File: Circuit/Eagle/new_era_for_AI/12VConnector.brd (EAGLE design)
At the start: 55.7 x 27.8 mm, 12 parts

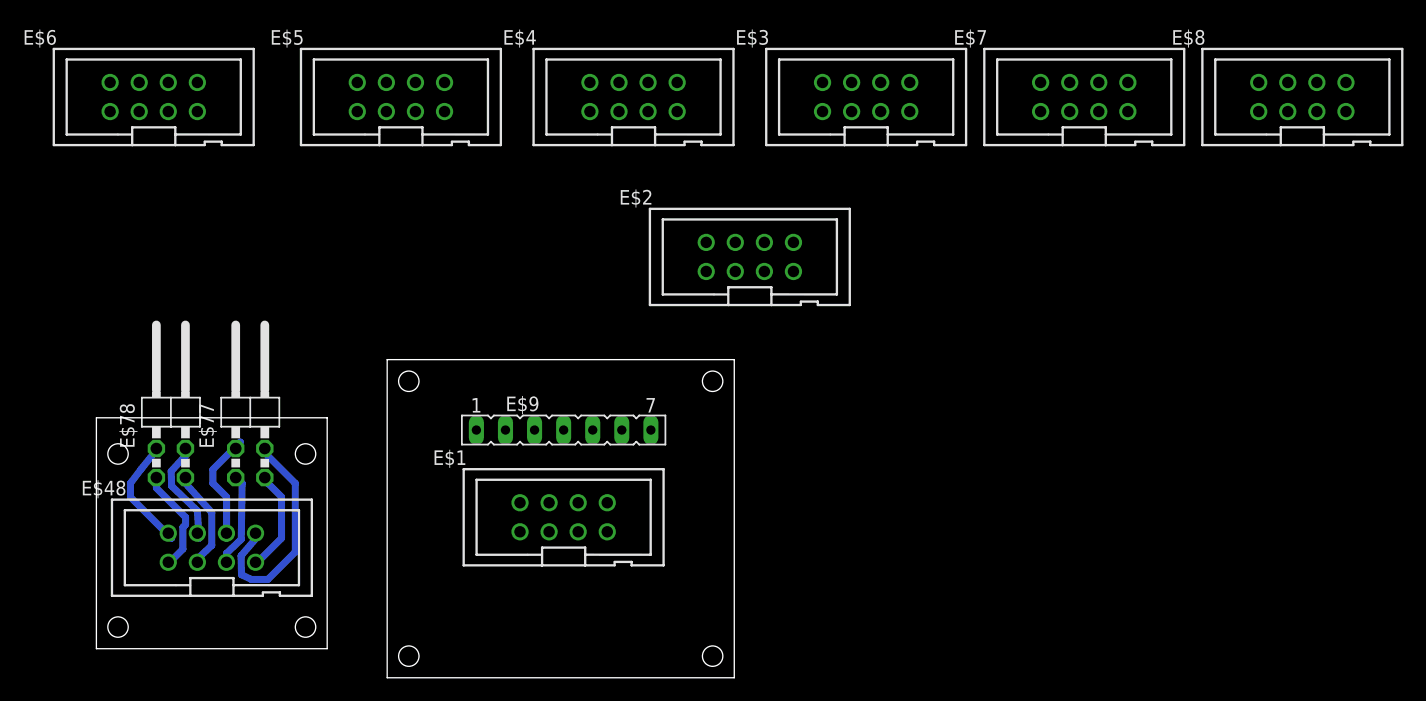
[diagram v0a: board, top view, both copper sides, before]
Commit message: .
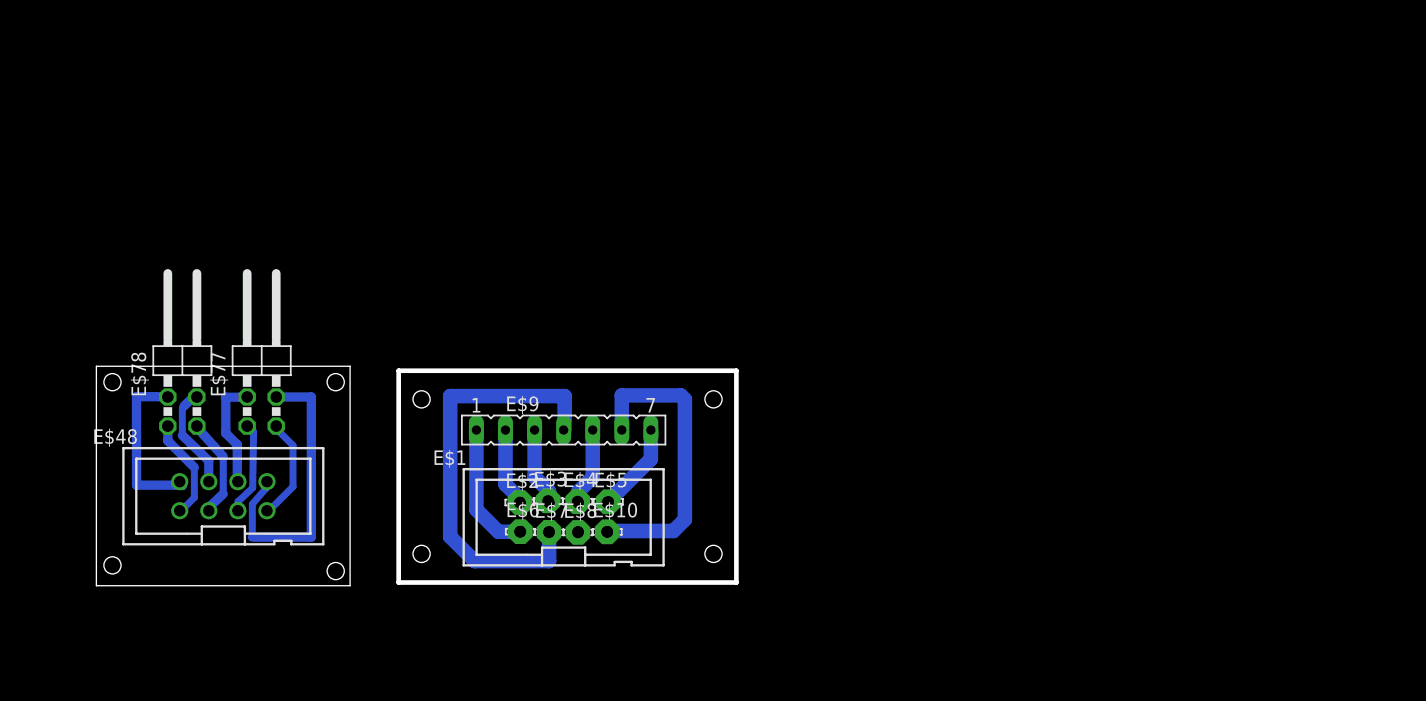
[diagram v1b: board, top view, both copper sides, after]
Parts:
- added E$10: (no value), solpad:LSP10
- E$2, E$3, E$4, E$5, E$6, E$7, E$8: device con-3m:PAK100/2500-8 -> solpad:LSP10
- moved E$8 72.7 mm to (43.2, 11.4)
- moved E$7 59.3 mm to (40.6, 11.4)
- moved E$6 50.5 mm to (38.1, 11.4)
- moved E$3 44.1 mm to (40.6, 14.1)
- moved E$5 40.3 mm to (45.8, 14.0)
- moved E$4 35.5 mm to (43.1, 14.1)
- moved E$2 28.5 mm to (38.1, 14.0)
- moved E$48 4.61 mm to (10.9, 14.5)
- moved E$77 4.61 mm to (15.5, 27.0)
- moved E$78 4.61 mm to (8.61, 27.0)
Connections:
- removed net S$11: E$2.10, E$7.9, E$8.10
- removed net S$12: E$2.9, E$8.9
- removed net S$13: E$2.8, E$3.9, E$7.10
- removed net S$8: E$2.5, E$3.10
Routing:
- net S$5: track 0.00 -> 37.4 mm
- net S$3: track 0.00 -> 26.4 mm
- net S$10: track 0.00 -> 11.6 mm
- net S$2: track 0.00 -> 7.93 mm
- net S$9: track 0.00 -> 6.88 mm
- net S$7: track 0.00 -> 6.88 mm
- net S$4: track 0.00 -> 6.88 mm
- net S$43: track 19.9 -> 25.7 mm
- net S$55: track 10.6 -> 15.3 mm
- net S$51: track 11.0 -> 9.69 mm
- net S$53: track 9.75 -> 9.09 mm
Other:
- board size 55.7 x 27.8 mm -> 55.9 x 19.2 mm
